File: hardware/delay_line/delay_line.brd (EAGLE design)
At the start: 56 x 28 mm, 36 parts, among them IC1 74AHC1G14DBV, IC2 74AHC1G14DBV, IC3 74AHC1G14DBV, IC4 74AHC1G14DBV, U1 DRV8836

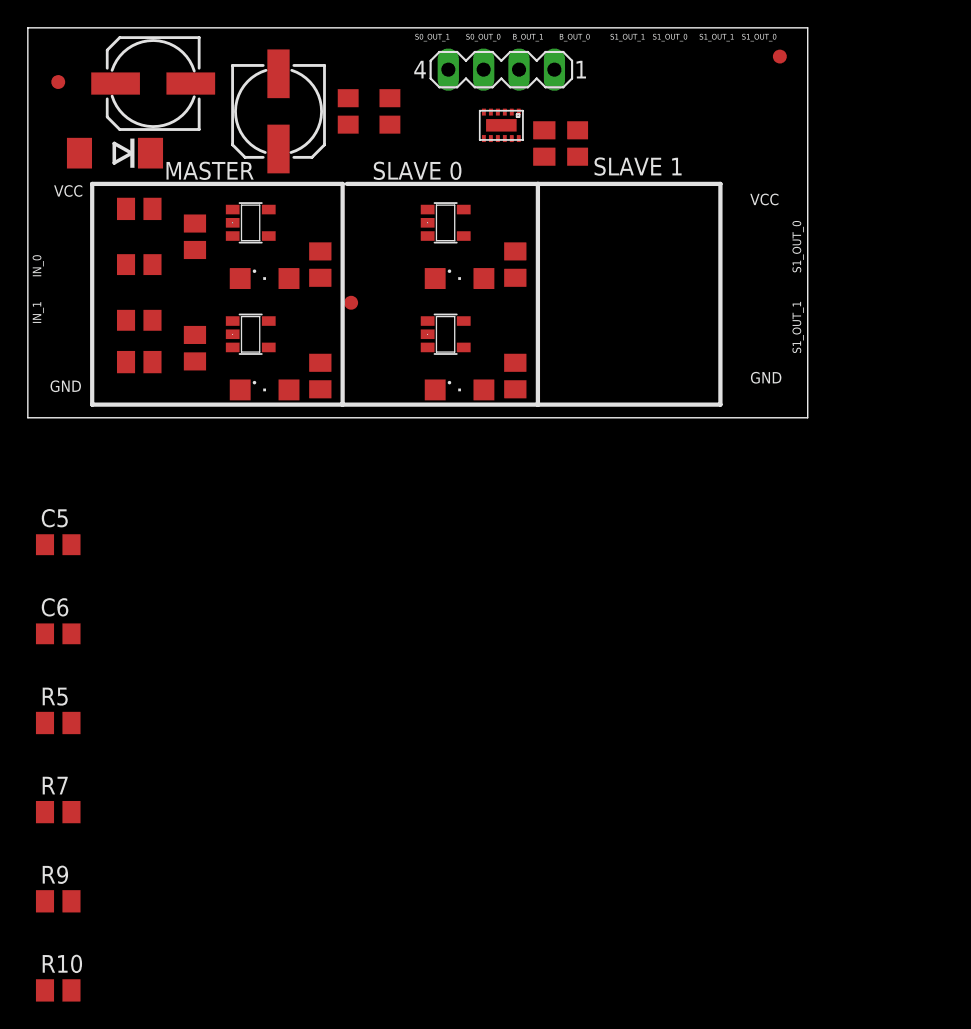
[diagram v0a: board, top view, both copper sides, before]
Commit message: board
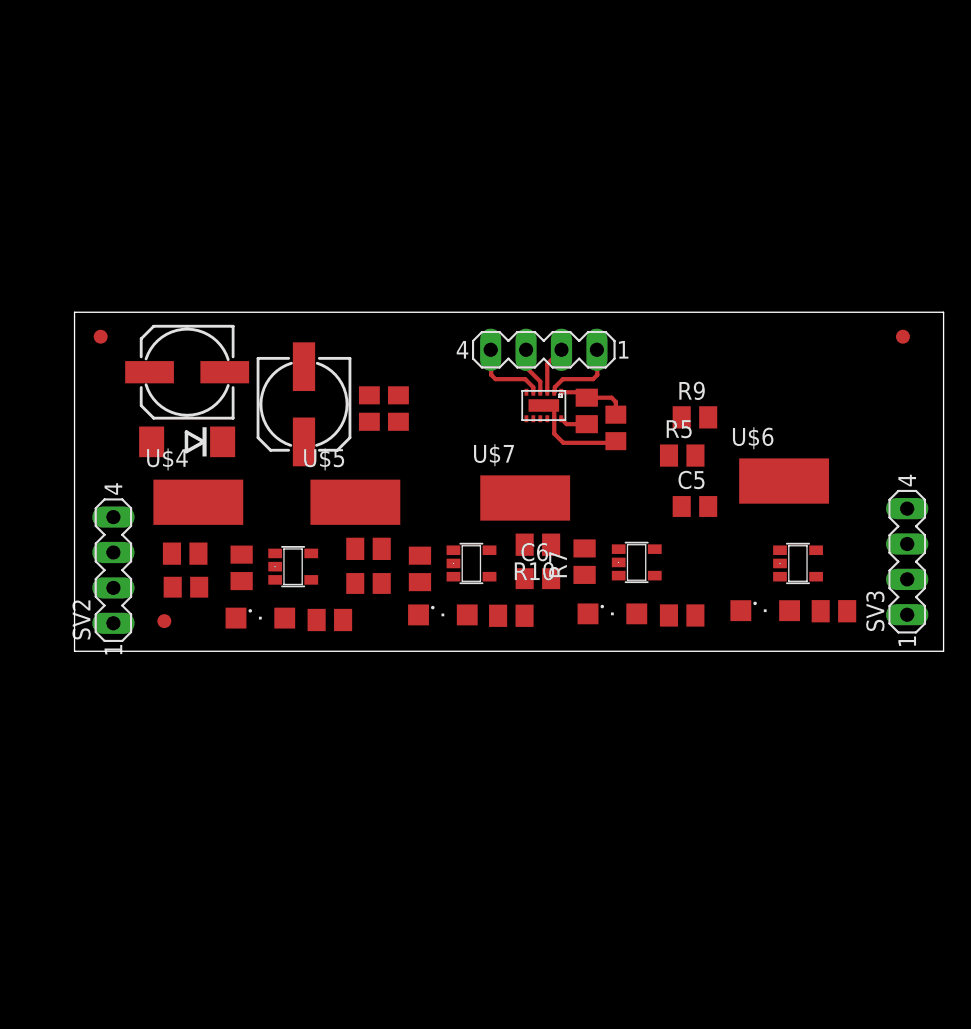
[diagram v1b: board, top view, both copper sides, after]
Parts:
- added SV2, SV3: (no value), con-lstb:MA04-1
- added U$4, U$5, U$6, U$7: SOLDER_PADNOSTOP, JCM:SOLDER_PAD_NOSTOP
- moved R9 57.4 mm to (50.9, 21.0)
- moved R5 48.7 mm to (50.0, 18.3)
- moved R10 47.0 mm to (39.6, 11.9), turned to 180 degrees
- moved C5 45.8 mm to (50.9, 14.6)
- moved R7 41.9 mm to (43.0, 10.7), turned to 90 degrees
- moved C6 34.7 mm to (39.6, 9.45)
- moved IC4 30.2 mm to (58.3, 10.5)
- moved R8 28.4 mm to (60.9, 7.11), turned to 0 degrees
- moved IC3 28.0 mm to (46.7, 10.6)
- moved R6 27.9 mm to (50.0, 6.81), turned to 0 degrees
- moved LED4 27.1 mm to (55.9, 7.15)
- moved U$3 26.5 mm to (12.8, 6.40)
- moved LED3 26.5 mm to (45.0, 6.92)
- moved R2 25.5 mm to (24.7, 6.48), turned to 0 degrees
- moved C4 25.1 mm to (27.5, 9.10)
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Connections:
- removed net B_OUT_0: C4.1, C5.1, IC1.4, R2.2, U1.10
- removed net B_OUT_1: C6.1, IC2.4, R4.2, U1.9
- removed net N$10: R9.2
- removed net N$12: R10.2
- removed net S0_OUT_0: IC3.4, R6.2, U1.8
- removed net S0_OUT_1: IC4.4, R8.2, U1.7
- new net IN_2: R9.2, U$6.SPAD
- new net IN_3: R10.2, U$7.SPAD
- new net OUT_0: C4.1, IC1.4, R2.2, U1.10
- new net OUT_1: C5.1, IC2.4, R4.2, U1.8
- new net OUT_2: C6.1, IC3.4, R6.2, U1.9
- new net OUT_3: IC4.4, R8.2, SV3.2, SV3.3, U1.7
- net GND: now also SV2.4, SV3.4
- net IN: now also SV2.2
- net IN_0: now also U$4.SPAD
- net IN_1: now also U$5.SPAD
- net VCC: now also SV2.1, SV3.1
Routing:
- net GND: track 0.00 -> 7.45 mm
- net N$34: track 0.00 -> 5.62 mm
- net N$30: track 0.00 -> 5.57 mm
- net VCC: track 0.00 -> 5.13 mm
- net N$31: track 0.00 -> 3.53 mm
- net N$33: track 0.00 -> 3.47 mm
- net N$32: track 0.00 -> 2.00 mm
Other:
- board size 56 x 28 mm -> 62.4 x 24.3 mm
- board text removed: "B_OUT_0"
- board text removed: "B_OUT_1"
- board text removed: "GND"
- board text removed: "IN_0"
- board text removed: "IN_1"
- board text removed: "MASTER"
- board text removed: "S0_OUT_0"
- board text removed: "S0_OUT_1"
- board text removed: "S1_OUT_0"
- board text removed: "S1_OUT_1"
- board text removed: "SLAVE 0"
- board text removed: "SLAVE 1"
- board text removed: "VCC"
